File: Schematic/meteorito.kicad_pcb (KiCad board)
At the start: 2 copper layers, 80 x 66.1 mm, 8 parts, among them P1 DH22, P2 GY-ML8511, P3 BMP180, P4 CONN_01X08, P5 CONN_01X08

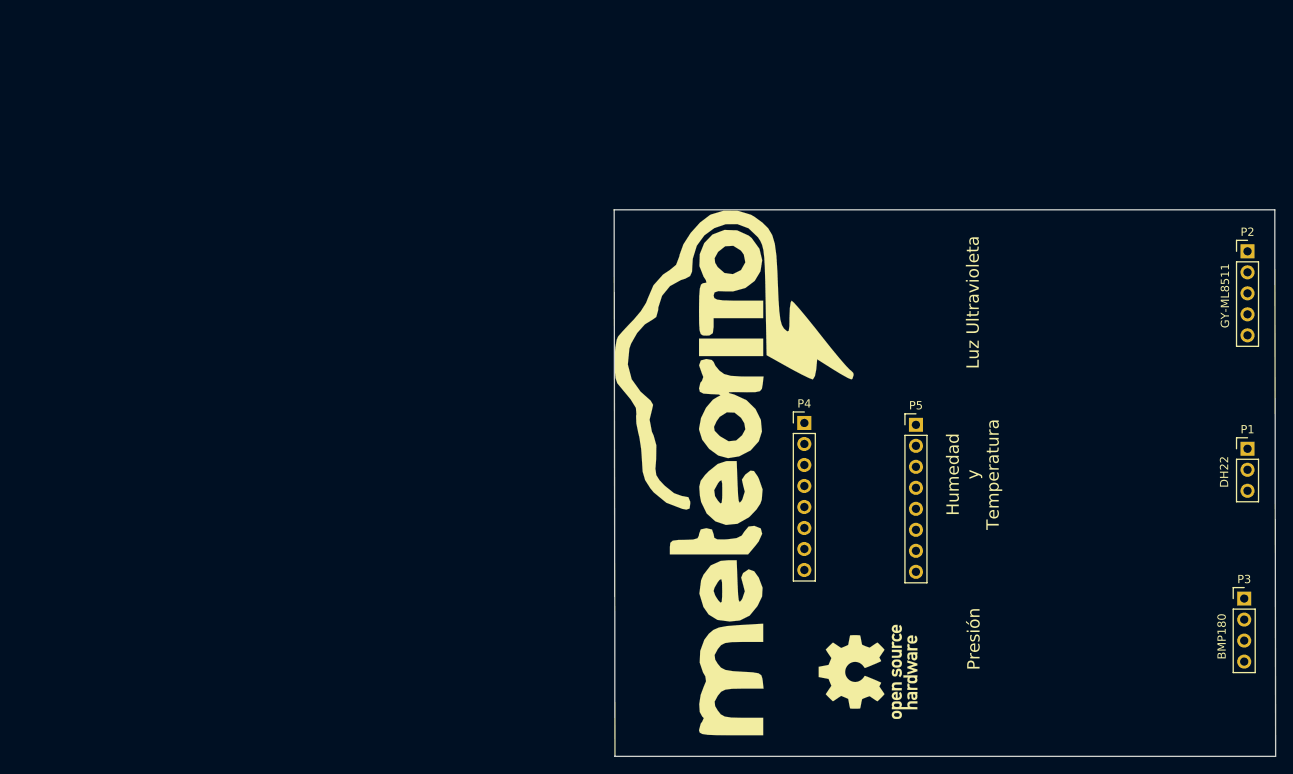
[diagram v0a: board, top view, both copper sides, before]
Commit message: Definicion de PCB
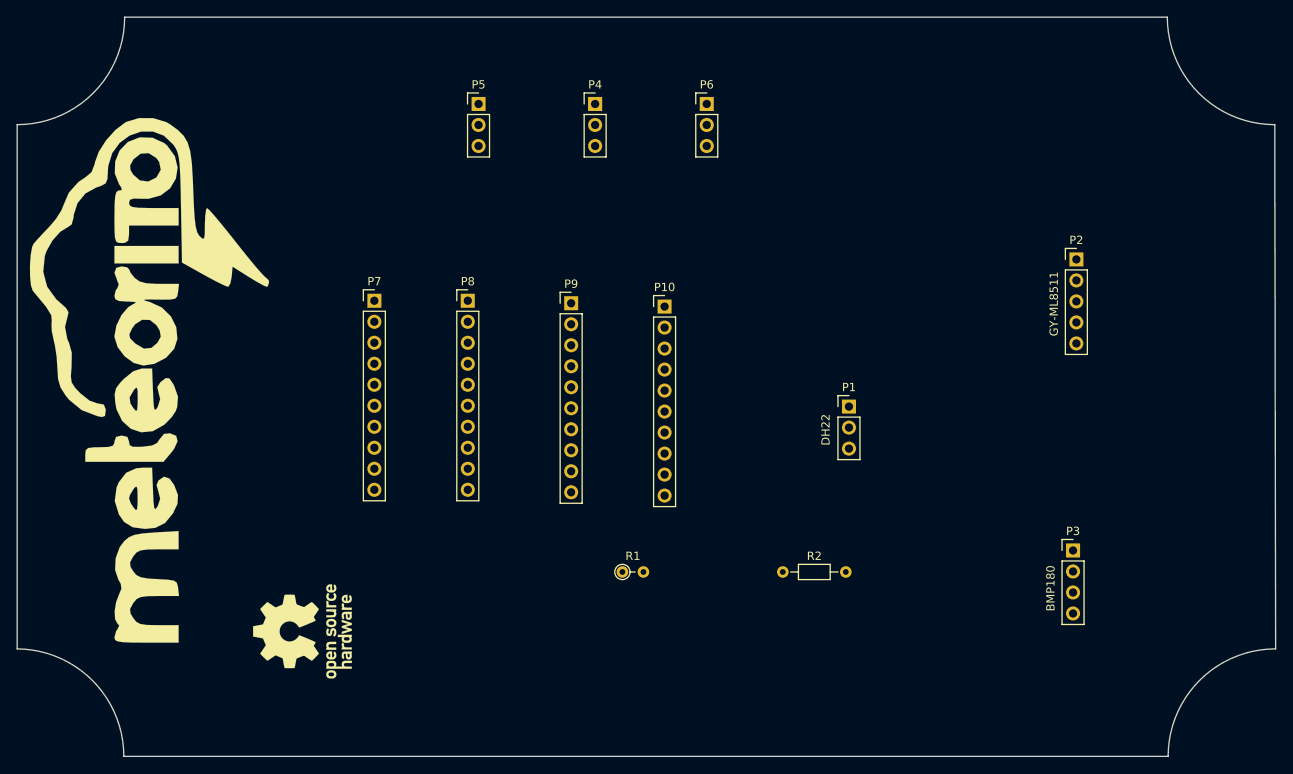
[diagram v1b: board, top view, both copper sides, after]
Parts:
- added P10: CONN_01X10, Connector_PinHeader_2.54mm:PinHeader_1x10_P2.54mm_Vertical, F.Cu at (118.1, 90.7)
- added P6: Hall, Connector_PinHeader_2.54mm:PinHeader_1x03_P2.54mm_Vertical, F.Cu at (123.2, 66.2)
- added P7: CONN_01X10, Connector_PinHeader_2.54mm:PinHeader_1x10_P2.54mm_Vertical, F.Cu at (83.0, 90.0)
- added P8: CONN_01X10, Connector_PinHeader_2.54mm:PinHeader_1x10_P2.54mm_Vertical, F.Cu at (94.3, 90.0)
- added P9: CONN_01X10, Connector_PinHeader_2.54mm:PinHeader_1x10_P2.54mm_Vertical, F.Cu at (106.8, 90.3)
- added R1: FOTORESISTENCIA, Resistor_THT:R_Axial_DIN0204_L3.6mm_D1.6mm_P2.54mm_Vertical, F.Cu at (113.0, 122.8)
- added R2: 100, Resistor_THT:R_Axial_DIN0204_L3.6mm_D1.6mm_P7.62mm_Horizontal, F.Cu at (132.4, 122.8)
- P4, P5: value CONN_01X08 -> Hall; footprint Pin_Headers:Pin_Header_Straight_1x08_Pitch2.54mm -> Connector_PinHeader_2.54mm:PinHeader_1x03_P2.54mm_Vertical
- moved G*** 90.4 mm to (74.7, 68.8)
- moved G*** 71.6 mm to (55.8, 99.6)
- moved REF*** 68.6 mm to (74.3, 130.0)
- moved P5 65.6 mm to (95.6, 66.2)
- moved P1 48.5 mm to (140.4, 102.8)
- moved P4 46.1 mm to (109.7, 66.2)
- moved P3 21.5 mm to (167.5, 120.2)
- moved P2 20.7 mm to (167.9, 85.0)
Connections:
- P1 pad 1: Net-(P1-Pad1) -> /IO23
- P1 pad 2: Net-(P1-Pad2) -> +5V
- P1 pad 3: Net-(P1-Pad3) -> GND
- P2 pad 1: Net-(P2-Pad1) -> +5V
- P2 pad 3: Net-(P2-Pad3) -> GND
- P2 pad 4: Net-(P2-Pad4) -> /IO27
- P2 pad 5: Net-(P2-Pad5) -> +5V
- P3 pad 1: Net-(P3-Pad1) -> +5V
- P3 pad 2: Net-(P3-Pad2) -> GND
- P3 pad 3: Net-(P3-Pad3) -> /IO22
- P3 pad 4: Net-(P3-Pad4) -> /IO21
- P4 pad 1: Net-(P4-Pad1) -> GND
- P4 pad 2: Net-(P4-Pad2) -> +5V
- P4 pad 3: Net-(P4-Pad3) -> /IO25
- P5 pad 1: Net-(P5-Pad1) -> GND
- P5 pad 2: Net-(P5-Pad2) -> +5V
- P5 pad 3: Net-(P5-Pad3) -> /IO17
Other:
- board size 80 x 66.1 mm -> 152.2 x 89.4 mm
- board text removed: "By"
- board text removed: "Humedad y Temperatura"
- board text removed: "Luz Ultravioleta"
- board text removed: "Presión"
- board text removed: "The Inventor's House"
- board text removed: "for"
